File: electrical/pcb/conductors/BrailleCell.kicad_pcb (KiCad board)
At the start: 2 copper layers, 6 x 11.5 mm, 9 parts, among them J1 Conn_01x08_Socket, J2 Conn_01x01_Pin, J3 Conn_01x01_Pin, J4 Conn_01x01_Pin, J5 Conn_01x01_Pin, J6 Conn_01x01_Pin, J7 Conn_01x01_Pin, J8 Conn_01x01_Pin, J9 Conn_01x01_Pin

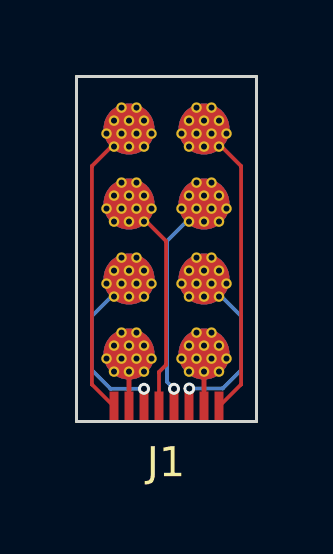
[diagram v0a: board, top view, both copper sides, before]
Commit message: library fix
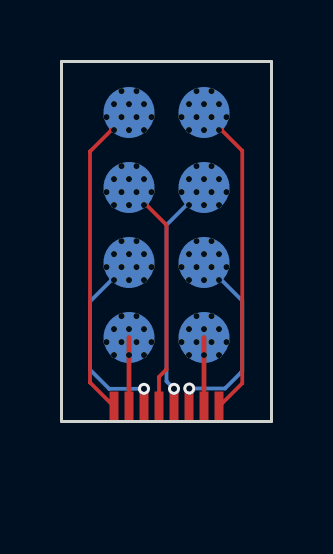
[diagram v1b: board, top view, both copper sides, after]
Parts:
- J2, J3, J4, J5, J6, J7, J8, J9: footprint BrailleLibrary:Pump Pin -> BrailleConnector:Pump Pin
- moved J2 0.55 mm to (151.8, 51.2)
- moved J3 0.55 mm to (151.8, 58.7)
- moved J4 0.55 mm to (151.8, 56.2)
- moved J5 0.55 mm to (151.8, 53.7)
- moved J6 0.55 mm to (154.2, 53.7)
- moved J7 0.55 mm to (154.2, 56.2)
- moved J8 0.55 mm to (154.2, 58.7)
- moved J9 0.55 mm to (154.2, 51.2)
- renumbered J1 to CONDUCTOR
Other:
- board size 6 x 11.5 mm -> 7 x 12 mm
